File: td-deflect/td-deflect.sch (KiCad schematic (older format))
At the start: 77 parts, among them J10 Conn_01x02_Male, J11 Conn_01x02_Male, J12 Conn_01x06_Male, J3 Conn_01x02_Male, Q1 BSC082N10LSG, Q10 IPD50R380CE, Q11 IPD50R380CE, Q2 C2M0045170D, Q3 BSC082N10LSG, Q4 BCP56, Q5 BCP53, Q6 BD139, Q7 BD140, Q8 IPD50R380CE, Q9 IPD50R380CE, T1 CST1, U1 MCP1416, U10 MIC4427, U5 TL082, U6 IRS2005S, U7 LTC6090, U8 INA181, U9 MIC4427

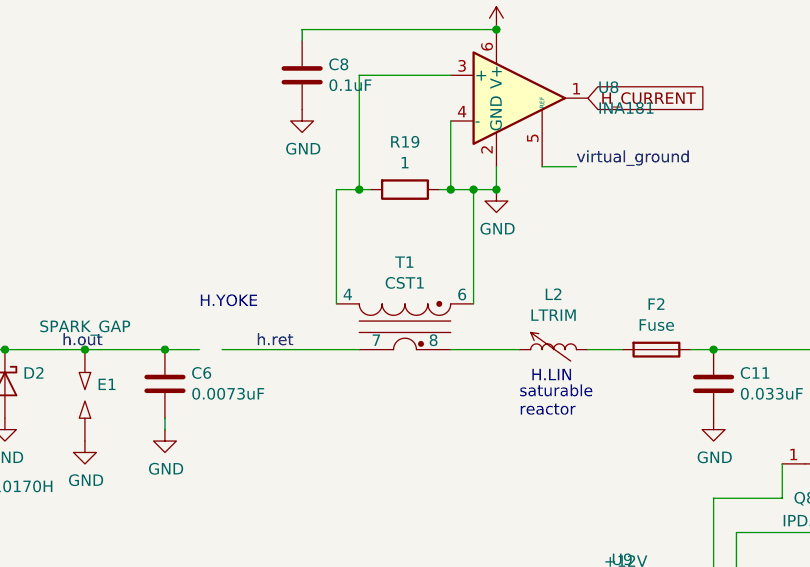
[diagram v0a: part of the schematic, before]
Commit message: asdf
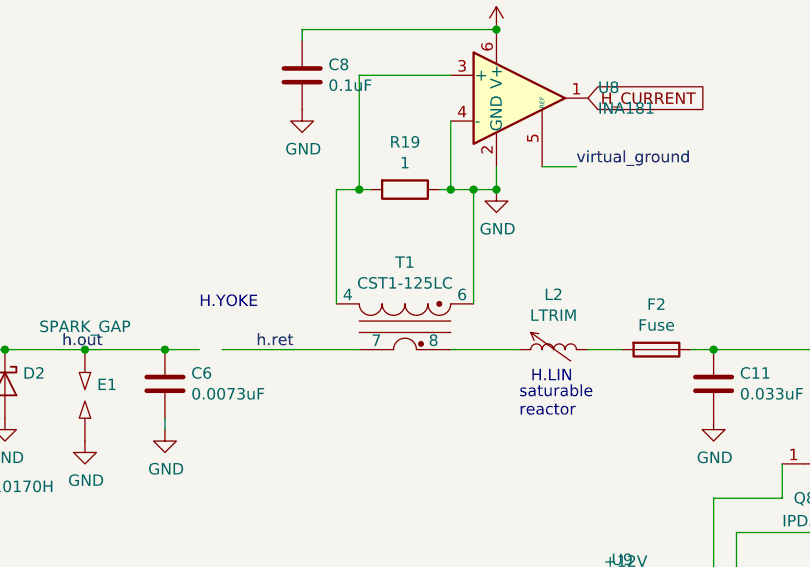
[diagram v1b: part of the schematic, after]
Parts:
- Q4: Digikey BCP56-16T1GOSCT-ND -> BCP56-16T1GOSCT-ND
- Q5: Digikey BCP53-16T1GOSCT-ND -> BCP53-16T1GOSCT-ND
- R1, R10, R11, R14, R17, R18, R19, R2, R22, R3, R5, R7, R8, R9: Digikey (none) -> 311-1.00CRCT-ND
- R12: Digikey BC4422CT-ND -> BC4422CT-ND
- R13, R15, R16: Digikey (none) -> 311-100CRCT-ND
- R20: Digikey (none) -> 311-220KCRCT-ND
- R21: Digikey (none) -> 311-1.00KCRCT-ND
- R23, R24, R25, R26, R27: Digikey (none) -> 311-100KFRCT-ND
- R28: Digikey (none) -> 311-1.00KFRCT-ND
- R4: Digikey (none) -> 311-0.01NUCT-ND
- T1: value CST1 -> CST1-125LC
- U1: Digikey (none) -> MCP1416T-E/OTCT-ND
- U10, U9: Digikey (none) -> 576-1525-5-ND
- U5: Digikey (none) -> 497-2212-1-ND
- U6: Digikey (none) -> IRS2005STRPBFCT-ND
- U7: Digikey (none) -> LTC6090CS8E-5#PBF-ND
- U8: Digikey (none) -> 296-47658-1-ND
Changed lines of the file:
@@
 F 2 "Package_TO_SOT_SMD:SOT-23-5" H 2300 2800 50  0001 C CIN
 F 3 "http://ww1.microchip.com/downloads/en/DeviceDoc/20002092F.pdf" H 2100 3450 50  0001 C CNN
+F 4 "MCP1416T-E/OTCT-ND" H 2300 3200 50  0001 C CNN "Digikey"
 	1    2300 3200
 	1    0    0    -1
@@
 F 2 "Resistor_SMD:R_0805_2012Metric_Pad1.15x1.40mm_HandSolder" V 2880 3200 50  0001 C CNN
 F 3 "~" H 2950 3200 50  0001 C CNN
+F 4 " 311-1.00CRCT-ND" H 2950 3200 50  0001 C CNN "Digikey"
 	1    2950 3200
 	0    1    1    0
@@
 F 2 "Resistor_SMD:R_0805_2012Metric_Pad1.15x1.40mm_HandSolder" V 3330 3550 50  0001 C CNN
 F 3 "~" H 3400 3550 50  0001 C CNN
+F 4 "311-0.01NUCT-ND" H 3400 3550 50  0001 C CNN "Digikey"
 	1    3400 3550
 	1    0    0    -1
@@
 F 3 "~" H 3850 3150 50  0001 C CNN
 F 4 "1700V" H 3850 3150 50  0001 C CNN "Voltage"
-F 5 " BC4422CT-ND " H 3850 3150 50  0001 C CNN "Digikey"
+F 5 "BC4422CT-ND" H 3850 3150 50  0001 C CNN "Digikey"
 	1    3850 3150
 	1    0    0    -1
@@
 F 2 "Package_SO:SOIC-8_3.9x4.9mm_P1.27mm" H 6900 4200 50  0001 C CNN
 F 3 "http://ww1.microchip.com/downloads/en/DeviceDoc/mic4426.pdf" H 6900 4200 50  0001 C CNN
+F 4 "576-1525-5-ND" H 6900 4500 50  0001 C CNN "Digikey"
 	1    6900 4500
 	1    0    0    -1
@@
 F 2 "Package_SO:SOIC-8_3.9x4.9mm_P1.27mm" H 8150 4200 50  0001 C CNN
 F 3 "http://ww1.microchip.com/downloads/en/DeviceDoc/mic4426.pdf" H 8150 4200 50  0001 C CNN
+F 4 "576-1525-5-ND" H 8150 4500 50  0001 C CNN "Digikey"
 	1    8150 4500
 	1    0    0    -1
@@
 F 2 "Resistor_SMD:R_0805_2012Metric_Pad1.15x1.40mm_HandSolder" V 2630 3350 50  0001 C CNN
 F 3 "~" H 2700 3350 50  0001 C CNN
+F 4 "311-1.00CRCT-ND" H 2700 3350 50  0001 C CNN "Digikey"
 	1    2700 3350
 	1    0    0    -1
@@
 F 2 "Resistor_SMD:R_0805_2012Metric_Pad1.15x1.40mm_HandSolder" V 1830 3350 50  0001 C CNN
 F 3 "~" H 1900 3350 50  0001 C CNN
+F 4 "311-1.00CRCT-ND" H 1900 3350 50  0001 C CNN "Digikey"
 	1    1900 3350
 	1    0    0    -1
@@
 F 2 "Resistor_SMD:R_1206_3216Metric_Pad1.42x1.75mm_HandSolder" V 7980 3500 50  0001 C CNN
 F 3 "~" H 8050 3500 50  0001 C CNN
+F 4 "311-100KFRCT-ND" H 8050 3500 50  0001 C CNN "Digikey"
 	1    8050 3500
 	1    0    0    -1
@@
 F 2 "Resistor_SMD:R_1206_3216Metric_Pad1.42x1.75mm_HandSolder" V 8530 3500 50  0001 C CNN
 F 3 "~" H 8600 3500 50  0001 C CNN
+F 4 "311-100KFRCT-ND" H 8600 3500 50  0001 C CNN "Digikey"
 	1    8600 3500
 	1    0    0    -1
@@
 F 2 "Resistor_SMD:R_1206_3216Metric_Pad1.42x1.75mm_HandSolder" V 9080 3500 50  0001 C CNN
 F 3 "~" H 9150 3500 50  0001 C CNN
+F 4 "311-100KFRCT-ND" H 9150 3500 50  0001 C CNN "Digikey"
 	1    9150 3500
 	1    0    0    -1
@@
 F 2 "Resistor_SMD:R_1206_3216Metric_Pad1.42x1.75mm_HandSolder" V 9630 3500 50  0001 C CNN
 F 3 "~" H 9700 3500 50  0001 C CNN
+F 4 "311-100KFRCT-ND" H 9700 3500 50  0001 C CNN "Digikey"
 	1    9700 3500
 	1    0    0    -1
@@
 F 2 "Resistor_SMD:R_0805_2012Metric_Pad1.15x1.40mm_HandSolder" V 5880 2300 50  0001 C CNN
 F 3 "~" H 5950 2300 50  0001 C CNN
+F 4 " 311-1.00CRCT-ND" H 5950 2300 50  0001 C CNN "Digikey"
 	1    5950 2300
 	0    1    1    0
@@
 F 2 "Package_TO_SOT_SMD:SOT-23-6" H 6500 1950 50  0001 C CNN
 F 3 "http://www.ti.com/lit/ds/symlink/ina181.pdf" H 6600 2050 50  0001 C CNN
+F 4 "296-47658-1-ND" H 6450 1900 50  0001 C CNN "Digikey"
 	1    6450 1900
 	1    0    0    -1
@@
 P 5950 2800
 F 0 "T1" H 5950 2619 50  0000 C CNN
-F 1 "CST1" H 5950 2710 50  0000 C CNN
+F 1 "CST1-125LC" H 5950 2710 50  0000 C CNN
 F 2 "Transformer_SMD:Transformer_Coilcraft_CST1" H 5950 2800 50  0001 C CNN
 F 3 "https://www.coilcraft.com/pdfs/cst.pdf" H 5950 2800 50  0001 C CNN
@@
 F 2 "Package_SO:SOIC-8_3.9x4.9mm_P1.27mm" H 2400 1600 50  0001 C CIN
 F 3 "https://www.infineon.com/dgdl/Infineon-IRS2005S-DS-v02_00-EN.pdf?fileId=5546d462533600a4015364c4246229e1" H 2400 1600 50  0001 C CNN
+F 4 "IRS2005STRPBFCT-ND" H 2400 1600 50  0001 C CNN "Digikey"
 	1    2400 1600
 	1    0    0    -1
@@
 F 2 "Resistor_SMD:R_0805_2012Metric_Pad1.15x1.40mm_HandSolder" V 5380 5650 50  0001 C CNN
 F 3 "~" H 5450 5650 50  0001 C CNN
+F 4 "311-100CRCT-ND" H 5450 5650 50  0001 C CNN "Digikey"
 	1    5450 5650
 	1    0    0    -1
@@
 F 2 "Resistor_SMD:R_0805_2012Metric_Pad1.15x1.40mm_HandSolder" V 5680 5950 50  0001 C CNN
 F 3 "~" H 5750 5950 50  0001 C CNN
+F 4 " 311-1.00CRCT-ND" H 5750 5950 50  0001 C CNN "Digikey"
 	1    5750 5950
 	1    0    0    -1
@@
 F 2 "Resistor_SMD:R_0805_2012Metric_Pad1.15x1.40mm_HandSolder" V 5680 6250 50  0001 C CNN
 F 3 "~" H 5750 6250 50  0001 C CNN
+F 4 " 311-1.00CRCT-ND" H 5750 6250 50  0001 C CNN "Digikey"
 	1    5750 6250
 	1    0    0    -1
@@
 F 2 "Resistor_SMD:R_0805_2012Metric_Pad1.15x1.40mm_HandSolder" V 5380 6550 50  0001 C CNN
 F 3 "~" H 5450 6550 50  0001 C CNN
+F 4 "311-100CRCT-ND" H 5450 6550 50  0001 C CNN "Digikey"
 	1    5450 6550
 	1    0    0    -1
@@
 F 2 "Package_TO_SOT_SMD:SOT-223-3_TabPin2" H 5550 6825 50  0001 L CIN
 F 3 "http://www.onsemi.com/pub_link/Collateral/BCP53T1-D.PDF" H 5350 6900 50  0001 L CNN
-F 4 " BCP53-16T1GOSCT-ND " H 5350 6900 50  0001 C CNN "Digikey"
+F 4 "BCP53-16T1GOSCT-ND " H 5350 6900 50  0001 C CNN "Digikey"
 	1    5350 6900
 	1    0    0    -1
@@
 F 2 "Package_TO_SOT_SMD:SOT-223-3_TabPin2" H 5550 5225 50  0001 L CIN
 F 3 "http://cache.nxp.com/documents/data_sheet/BCP56_BCX56_BC56PA.pdf?pspll=1" H 5350 5300 50  0001 L CNN
-F 4 " BCP56-16T1GOSCT-ND " H 5350 5300 50  0001 C CNN "Digikey"
+F 4 "BCP56-16T1GOSCT-ND " H 5350 5300 50  0001 C CNN "Digikey"
 	1    5350 5300
 	1    0    0    -1
@@
 F 2 "Package_SO:SOIC-8-1EP_3.9x4.9mm_P1.27mm_EP2.29x3mm" H 3800 6100 50  0001 C CNN
 F 3 "" H 3800 6100 50  0001 C CNN
+F 4 "LTC6090CS8E-5#PBF-ND" H 3800 6100 50  0001 C CNN "Digikey"
 	1    3800 6100
 	1    0    0    -1
@@
 F 2 "Resistor_SMD:R_0805_2012Metric_Pad1.15x1.40mm_HandSolder" V 5230 6100 50  0001 C CNN
 F 3 "~" H 5300 6100 50  0001 C CNN
+F 4 "311-1.00CRCT-ND" H 5300 6100 50  0001 C CNN "Digikey"
 	1    5300 6100
 	0    -1   -1   0
@@
 F 2 "Resistor_SMD:R_0805_2012Metric_Pad1.15x1.40mm_HandSolder" V 4630 6100 50  0001 C CNN
 F 3 "~" H 4700 6100 50  0001 C CNN
+F 4 "311-100CRCT-ND" H 4700 6100 50  0001 C CNN "Digikey"
 	1    4700 6100
 	0    1    1    0
@@
 F 2 "Resistor_SMD:R_0805_2012Metric_Pad1.15x1.40mm_HandSolder" V 6580 6350 50  0001 C CNN
 F 3 "~" H 6650 6350 50  0001 C CNN
+F 4 " 311-1.00CRCT-ND" H 6650 6350 50  0001 C CNN "Digikey"
 	1    6650 6350
 	1    0    0    -1
@@
 F 2 "Resistor_SMD:R_0805_2012Metric_Pad1.15x1.40mm_HandSolder" V 6130 6550 50  0001 C CNN
 F 3 "~" H 6200 6550 50  0001 C CNN
+F 4 " 311-220KCRCT-ND" H 6200 6550 50  0001 C CNN "Digikey"
 	1    6200 6550
 	1    0    0    -1
@@
 F 2 "Resistor_SMD:R_0805_2012Metric_Pad1.15x1.40mm_HandSolder" V 6280 7150 50  0001 C CNN
 F 3 "~" H 6350 7150 50  0001 C CNN
+F 4 " 311-1.00KCRCT-ND" H 6350 7150 50  0001 C CNN "Digikey"
 	1    6350 7150
 	0    1    1    0
@@
 F 2 "Package_SO:SOIC-8_3.9x4.9mm_P1.27mm" H 2950 6000 50  0001 C CNN
 F 3 "http://www.ti.com/lit/ds/symlink/tl081.pdf" H 2950 6000 50  0001 C CNN
+F 4 "497-2212-1-ND" H 2750 6000 50  0001 C CNN "Digikey"
 	2    2750 6000
 	1    0    0    -1
@@
 F 2 "Package_SO:SOIC-8_3.9x4.9mm_P1.27mm" H 1100 6350 50  0001 C CNN
 F 3 "http://www.ti.com/lit/ds/symlink/tl081.pdf" H 1100 6350 50  0001 C CNN
+F 4 "497-2212-1-ND" H 1100 6350 50  0001 C CNN "Digikey"
 	3    1100 6350
 	1    0    0    -1
@@
 F 2 "Resistor_SMD:R_0805_2012Metric_Pad1.15x1.40mm_HandSolder" V 2680 6400 50  0001 C CNN
 F 3 "~" H 2750 6400 50  0001 C CNN
+F 4 "311-1.00CRCT-ND" H 2750 6400 50  0001 C CNN "Digikey"
 	1    2750 6400
 	0    -1   -1   0
@@
 F 2 "Resistor_SMD:R_0805_2012Metric_Pad1.15x1.40mm_HandSolder" V 2230 6400 50  0001 C CNN
 F 3 "~" H 2300 6400 50  0001 C CNN
+F 4 "311-1.00CRCT-ND" H 2300 6400 50  0001 C CNN "Digikey"
 	1    2300 6400
 	0    1    1    0
@@
 F 2 "Resistor_SMD:R_0805_2012Metric_Pad1.15x1.40mm_HandSolder" V 1330 6150 50  0001 C CNN
 F 3 "~" H 1400 6150 50  0001 C CNN
+F 4 "311-1.00CRCT-ND" H 1400 6150 50  0001 C CNN "Digikey"
 	1    1400 6150
 	1    0    0    -1
@@
 F 2 "Resistor_SMD:R_0805_2012Metric_Pad1.15x1.40mm_HandSolder" V 1330 6450 50  0001 C CNN
 F 3 "~" H 1400 6450 50  0001 C CNN
+F 4 "311-1.00CRCT-ND" H 1400 6450 50  0001 C CNN "Digikey"
 	1    1400 6450
 	1    0    0    -1
@@
 F 2 "Resistor_SMD:R_0805_2012Metric_Pad1.15x1.40mm_HandSolder" V 2080 5750 50  0001 C CNN
 F 3 "~" H 2150 5750 50  0001 C CNN
+F 4 "311-1.00CRCT-ND" H 2150 5750 50  0001 C CNN "Digikey"
 	1    2150 5750
 	1    0    0    -1
@@
 F 2 "Resistor_SMD:R_0805_2012Metric_Pad1.15x1.40mm_HandSolder" V 1930 5600 50  0001 C CNN
 F 3 "~" H 2000 5600 50  0001 C CNN
+F 4 "311-1.00CRCT-ND" H 2000 5600 50  0001 C CNN "Digikey"
 	1    2000 5600
 	0    1    1    0
@@
 F 3 "~" H 10250 3150 50  0001 C CNN
 F 4 "200V" H 10250 3150 50  0001 C CNN "Voltage"
+F 5 "311-100KFRCT-ND" H 10250 3150 50  0001 C CNN "Digikey"
 	1    10250 3150
 	1    0    0    -1
@@
 F 3 "~" H 10250 3550 50  0001 C CNN
 F 4 "200V" H 10250 3550 50  0001 C CNN "Voltage"
+F 5 " 311-1.00KFRCT-ND" H 10250 3550 50  0001 C CNN "Digikey"
 	1    10250 3550
 	1    0    0    -1
@@
 F 2 "Package_SO:SOIC-8_3.9x4.9mm_P1.27mm" H 1850 6400 50  0001 C CNN
 F 3 "http://www.ti.com/lit/ds/symlink/tl081.pdf" H 1850 6400 50  0001 C CNN
+F 4 "497-2212-1-ND" H 1850 6400 50  0001 C CNN "Digikey"
 	1    1850 6400
 	1    0    0    -1
